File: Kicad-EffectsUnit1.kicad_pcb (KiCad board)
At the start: 2 copper layers, 100 x 100 mm, 166 parts, among them J101 In7, J102 Doepfer connector, J103 Vin 7-12v, J104 In6, J105 In3, J106 Out10, J107 Out11, J108 Out12, J109 Out13, J110 Power Conn, J201 In, J202 Out, P201 HEADER_2x5_Doepfer, Q201 BC337, Q202 PZT2222A, Q203 PZT2222A, SW101 Dist 10, SW102 Crush A3, SW103 Rotary_Encoder_Switch, SW104 Dist 12, U101 TL072, U102 TL072, U201 TL072, U202 PT2399

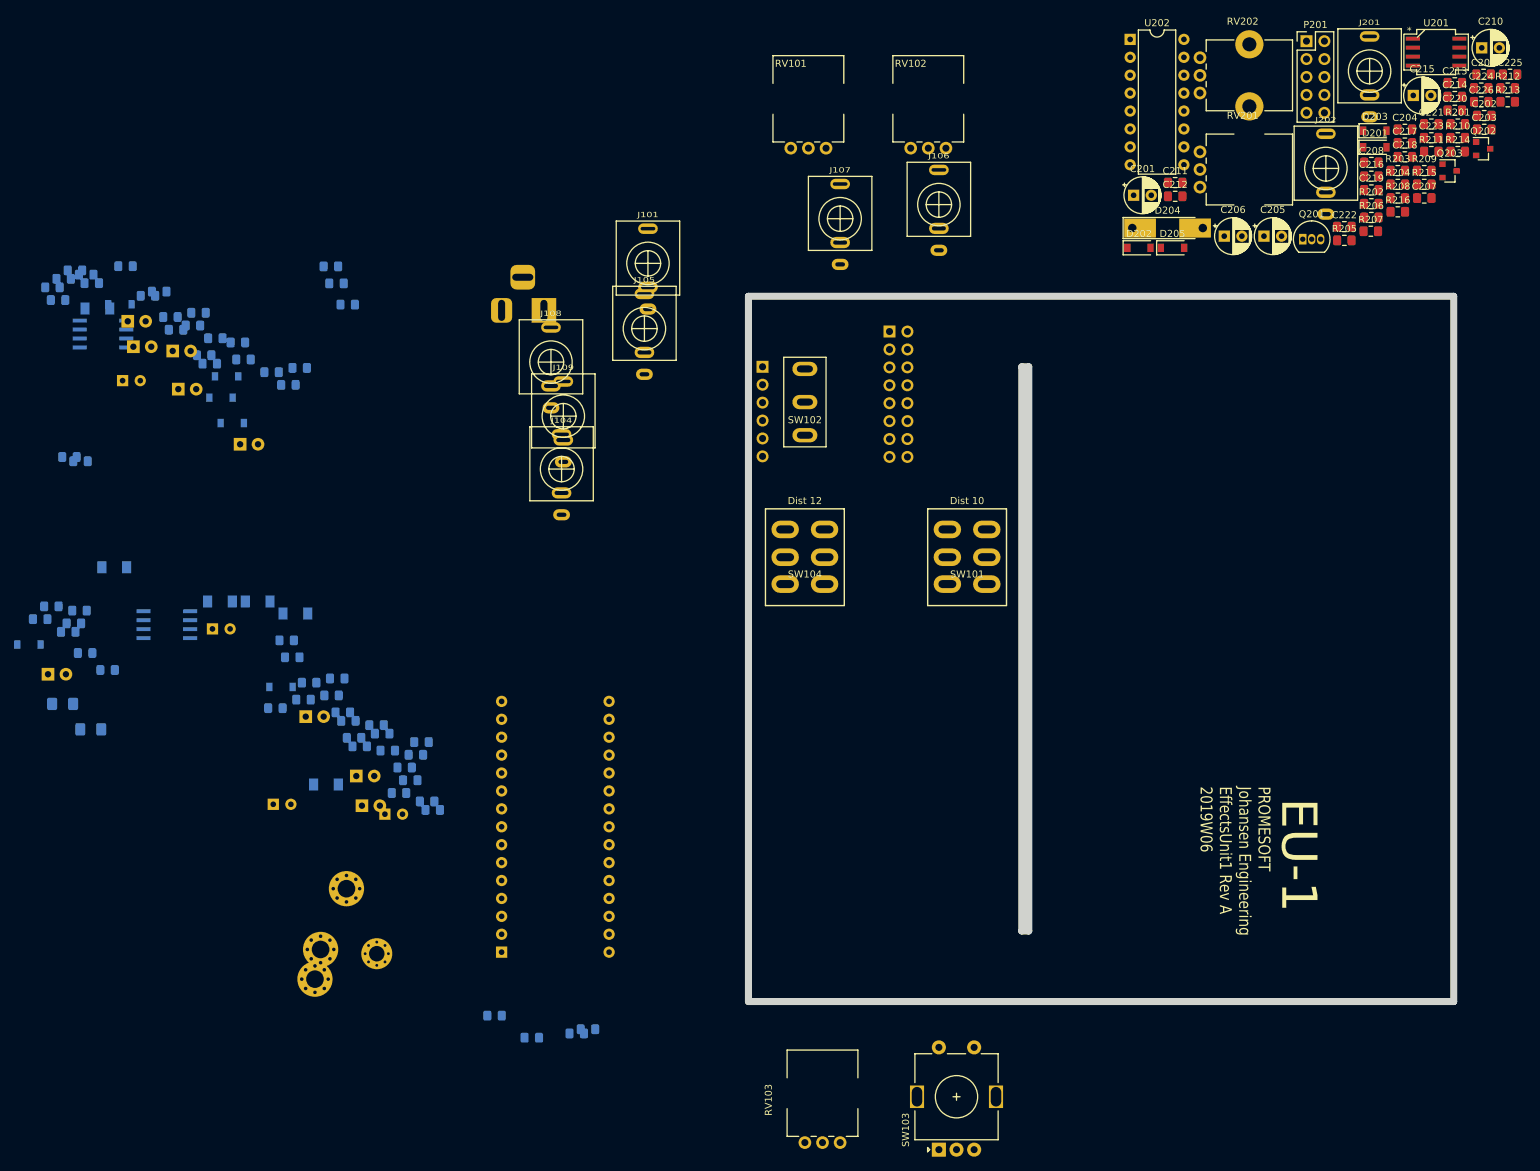
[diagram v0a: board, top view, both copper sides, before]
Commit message: PCB work
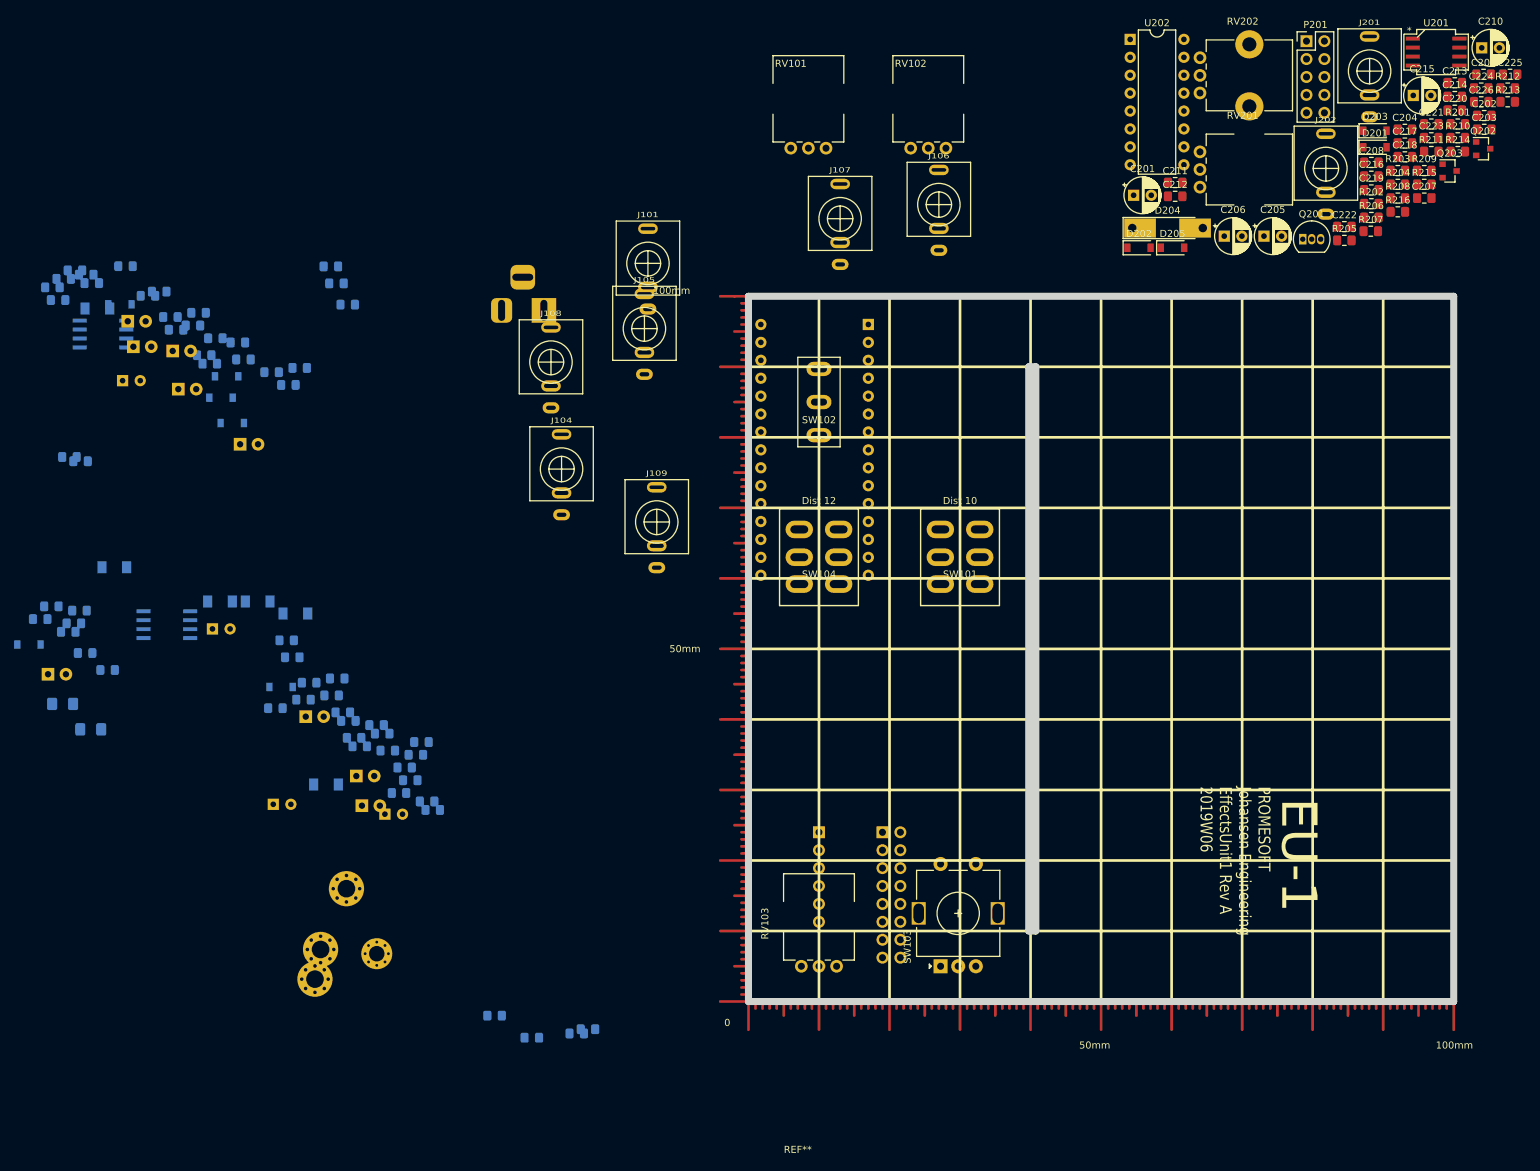
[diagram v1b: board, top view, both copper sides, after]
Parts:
- added REF**: Gauge_100mm_Grid_Type1_Silk_CopperTop, AJ:Gauge_100mm_Grid_Type1_Silk_CopperTop, F.Cu at (100.0, 150.0)
- moved A101 103.1 mm to (117.0, 54.0), turned to 180 degrees
- moved J102 71.0 mm to (119.0, 126.0)
- moved J110 66.5 mm to (110.0, 126.0)
- moved SW103 26.0 mm to (127.2, 145.0)
- moved RV103 25.0 mm to (112.5, 145.0)
- moved J109 20.0 mm to (87.0, 82.0)
- moved SW102 2.00 mm to (110.0, 65.0)
- moved SW104 2.00 mm to (110.0, 87.0)
- moved SW101 1.00 mm to (130.0, 87.0)
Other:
- outline, holes or cut-outs redrawn
